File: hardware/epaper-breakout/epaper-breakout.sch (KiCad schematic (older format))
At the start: 59 parts, among them J1 XF2M-3315-1A, J2 C10418, J3 Conn_01x10, Q1 IRLML6402, U1 LT1086-3.3, U2 LT1945, U3 L7915, U4 L7815, U5 ESP32-WROOM-32, U6 CH330N, U7 LM358

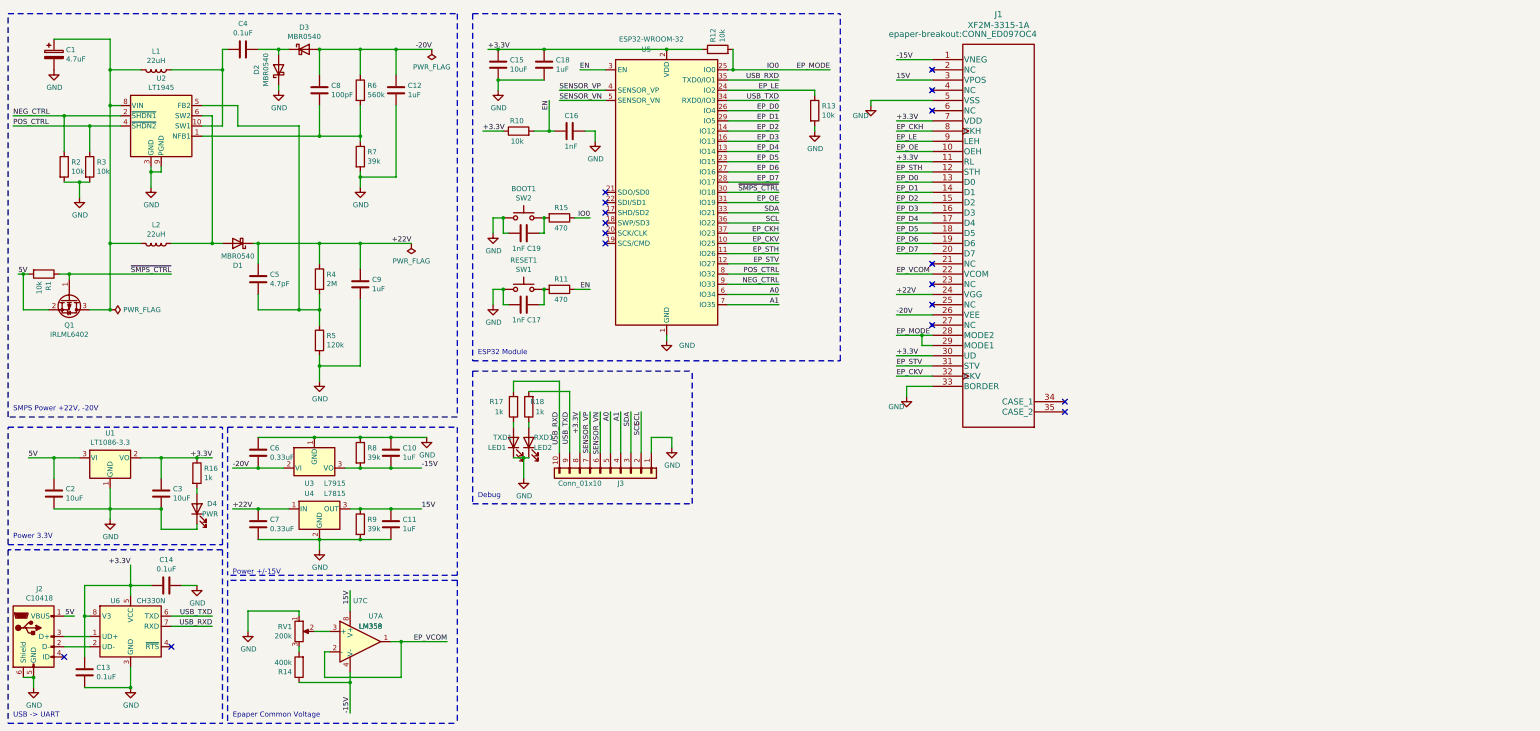
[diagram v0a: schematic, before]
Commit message: change to wrover module
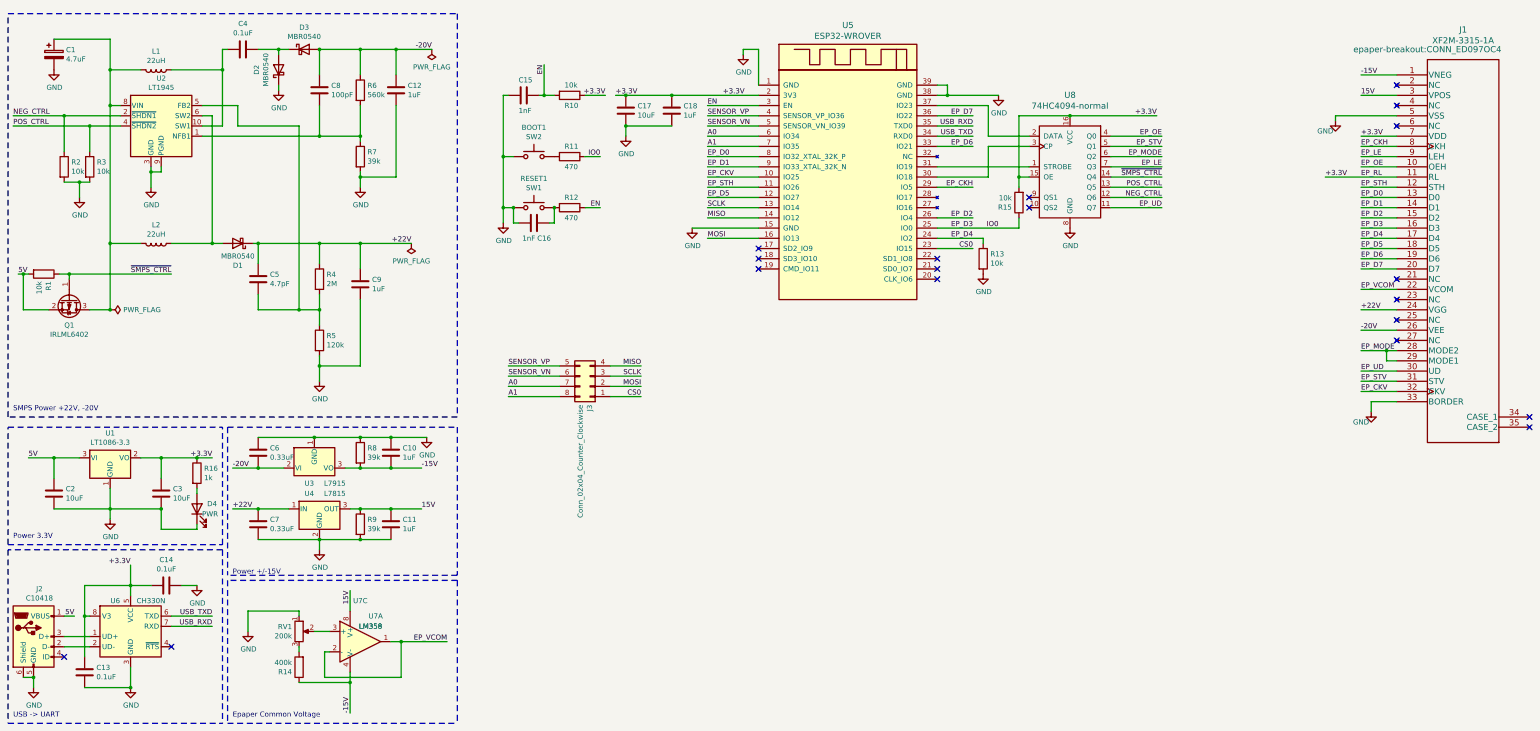
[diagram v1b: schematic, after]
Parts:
- removed C19: 1nF, Capacitor_SMD:C_0603_1608Metric, symbol Device:C
- removed J3: Conn_01x10, Connector_PinHeader_2.54mm:PinHeader_1x10_P2.54mm_Vertical, symbol Connector_Generic:Conn_01x10
- removed R17, R18: 1k, Resistor_SMD:R_0805_2012Metric, symbol Device:R
- removed RXD1: LED2, LED_SMD:LED_0805_2012Metric, symbol Device:LED
- removed TXD1: LED1, LED_SMD:LED_0805_2012Metric, symbol Device:LED
- removed U5: ESP32-WROOM-32, RF_Module:ESP32-WROOM-32, symbol RF_Module:ESP32-WROOM-32
- added J3: Conn_02x04_Counter_Clockwise, symbol Connector_Generic:Conn_02x04_Counter_Clockwise
- added U5: ESP32-WROVER, symbol esp32-wrover:ESP32-WROVER
- added U8: 74HC4094-normal, symbol 74HC4094:74HC4094-normal
- C15: value 10uF -> 1nF
- C17: value 1nF -> 10uF
- R12: value 10k -> 470
- R15: value 470 -> 10k
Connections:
- net +3.3V: now also C17.1, R15.2, U5.2 (3V3), U8.15 (OE), U8.16 (VCC); no longer C15.1, J1.30 (UD), R12.1
- net A0: now also J3.7 (Pin_7), U5.6 (IO34)
- net A1: now also J3.8 (Pin_8), U5.7 (IO35)
- net EN: now also C15.2, R12.1, U5.3 (EN); no longer C16.1, R11.1
- net EP_CKH: now also U5.29 (IO5)
- net EP_CKV: now also U5.10 (IO25)
- net EP_D0: now also U5.8 (IO32_XTAL_32K_P)
- net EP_D1: now also U5.9 (IO33_XTAL_32K_N)
- net EP_D2: now also U5.26 (IO4)
- net EP_D3: now also R11.1, R15.1, U5.25 (IO0)
- net EP_D4: now also R13.1, U5.24 (IO2)
- net EP_D5: now also U5.12 (IO27)
- net EP_D6: now also U5.33 (IO21)
- net EP_D7: now also U5.36 (IO22)
- net EP_LE: now also U8.7 (Q3); no longer R13.1
- net EP_MODE: now also U8.6 (Q2); no longer R12.2, R15.1
- net EP_OE: now also U8.4 (Q0)
- net EP_STH: now also U5.11 (IO26)
- net EP_STV: now also U8.5 (Q1)
- net GND: now also C15.1, C16.1, C17.2, U5.1 (GND), U5.15 (GND), U5.38 (GND), U5.39 (GND), U8.8 (GND); no longer C15.2, C16.2, C17.1
- net NEG_CTRL: now also U8.12 (Q6)
- net POS_CTRL: now also U8.13 (Q5)
- net SENSOR_VN: now also J3.6 (Pin_6), U5.5 (SENSOR_VN_IO39)
- net SENSOR_VP: now also J3.5 (Pin_5), U5.4 (SENSOR_VP_IO36)
- net USB_RXD: now also U5.35 (TXD0)
- net USB_TXD: now also U5.34 (RXD0)
- net ~SMPS_CTRL: now also U8.14 (Q4)
- net at BOOT1.2: now also R11.2; no longer R15.2
- new net: U5.30 (IO18), U8.3 (CP)
- new net: U5.31 (IO19), U8.1 (STROBE)
- new net: U5.37 (IO23), U8.2 (DATA)
- new net: C16.2, R12.2, RESET1.2
- new net CS0: J3.1 (Pin_1), U5.23 (IO15)
- new net EP_UD: J1.30 (UD), U8.11 (Q7)
- new net MISO: J3.4 (Pin_4), U5.14 (IO12)
- new net MOSI: J3.2 (Pin_2), U5.16 (IO13)
- new net SCLK: J3.3 (Pin_3), U5.13 (IO14)
- no-connect marks 17 -> 19
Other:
- note removed: "Debug"
- note removed: "ESP32 Module"
- moved on the sheet: J1
